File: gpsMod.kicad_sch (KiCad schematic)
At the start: 29 parts, among them U2 MAX2769B, U3 MAX8510EXK29+T, U4 MAX8510EXK29+T, Y1 TXETCDSANF-16.368000

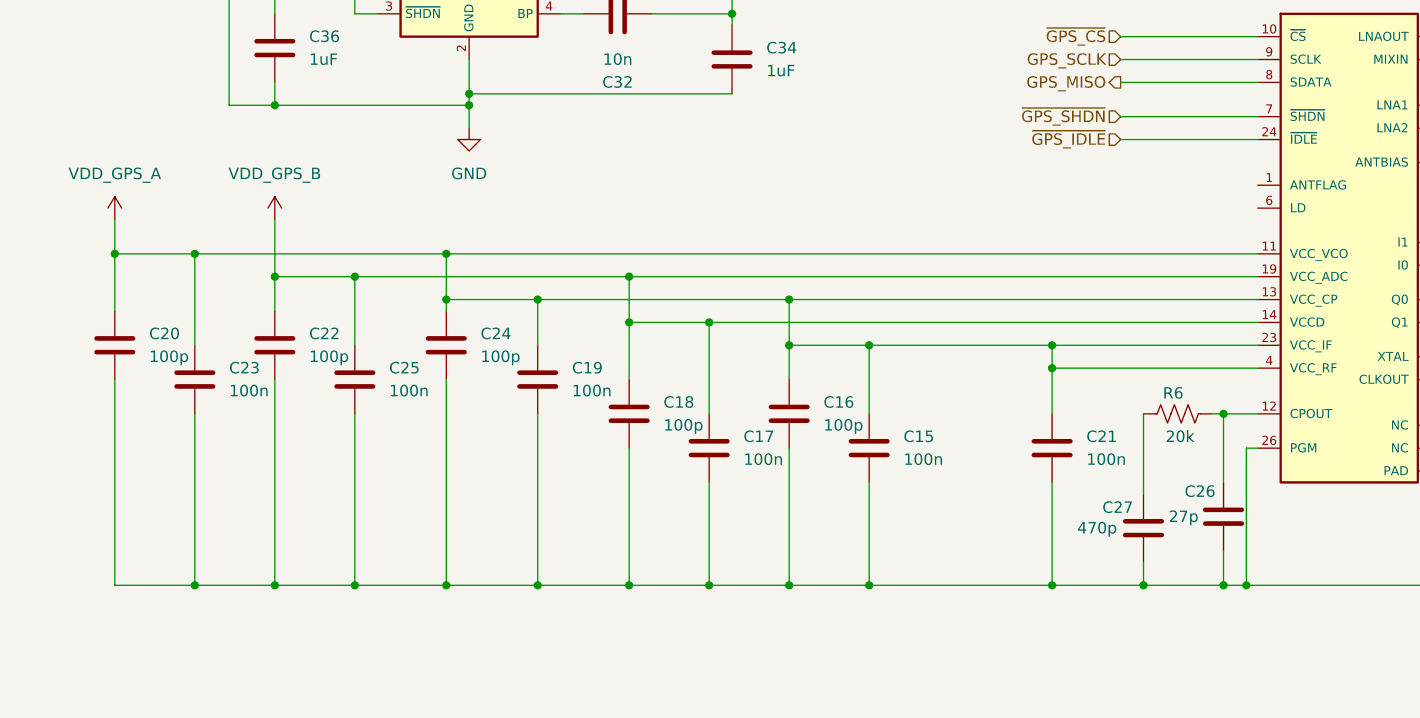
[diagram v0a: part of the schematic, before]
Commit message: starting to lay the board out.
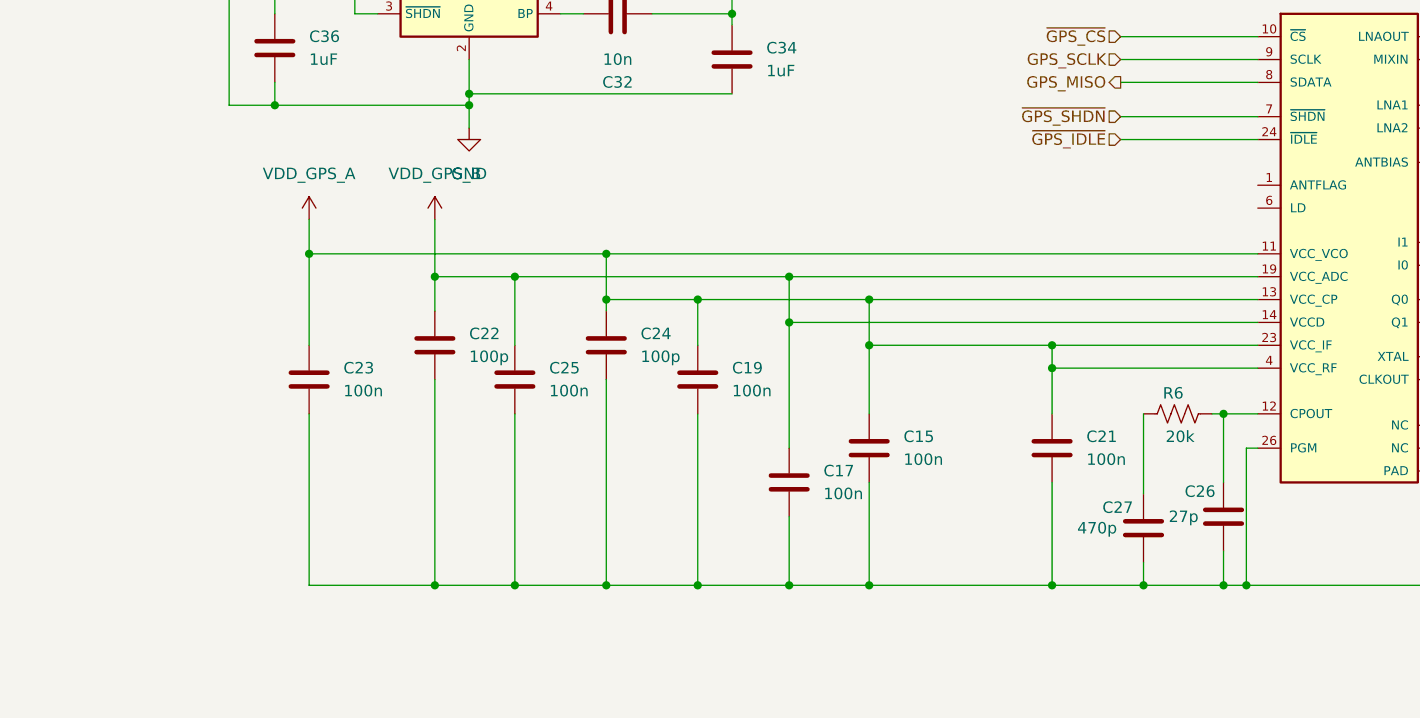
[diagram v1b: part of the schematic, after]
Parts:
- removed C16, C18, C20: 100p, AllardChip:CAPC60X30X33L15L, symbol AllardPassive:C10AB1-10000
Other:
- moved on the sheet: C17, C19, C22, C23, C24, C25
